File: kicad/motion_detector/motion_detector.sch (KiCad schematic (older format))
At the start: 15 parts

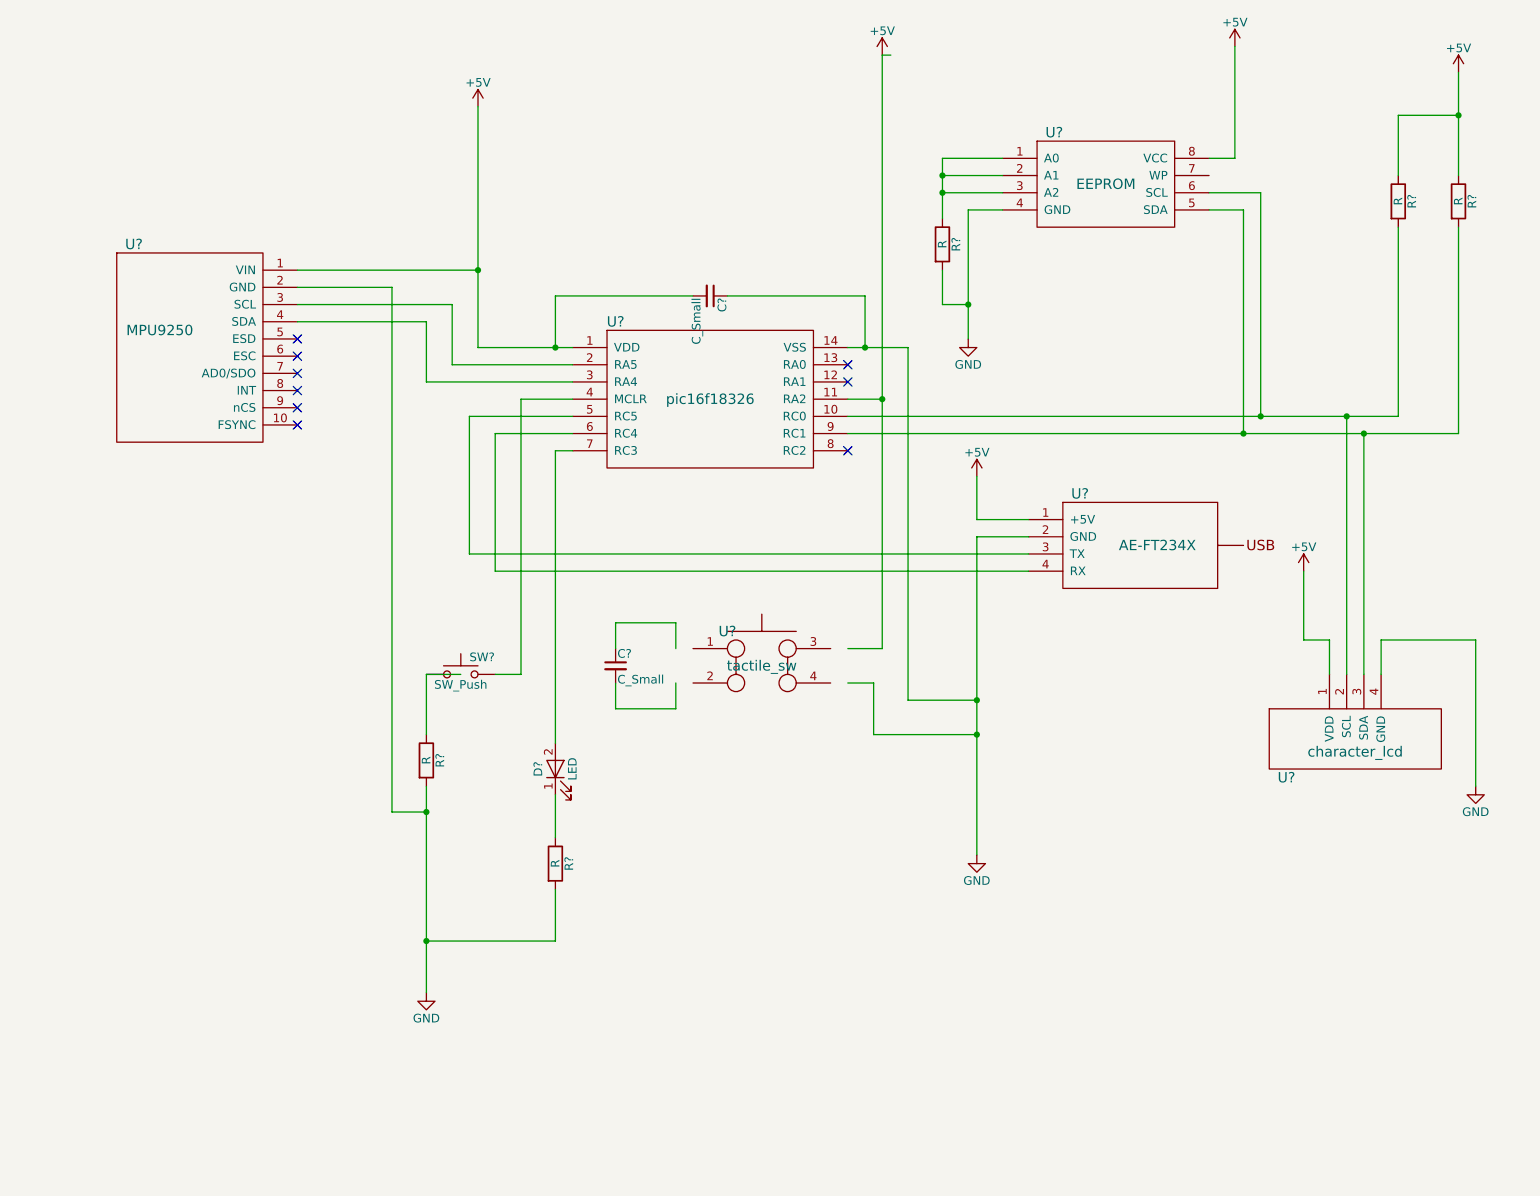
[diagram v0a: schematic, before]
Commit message: update
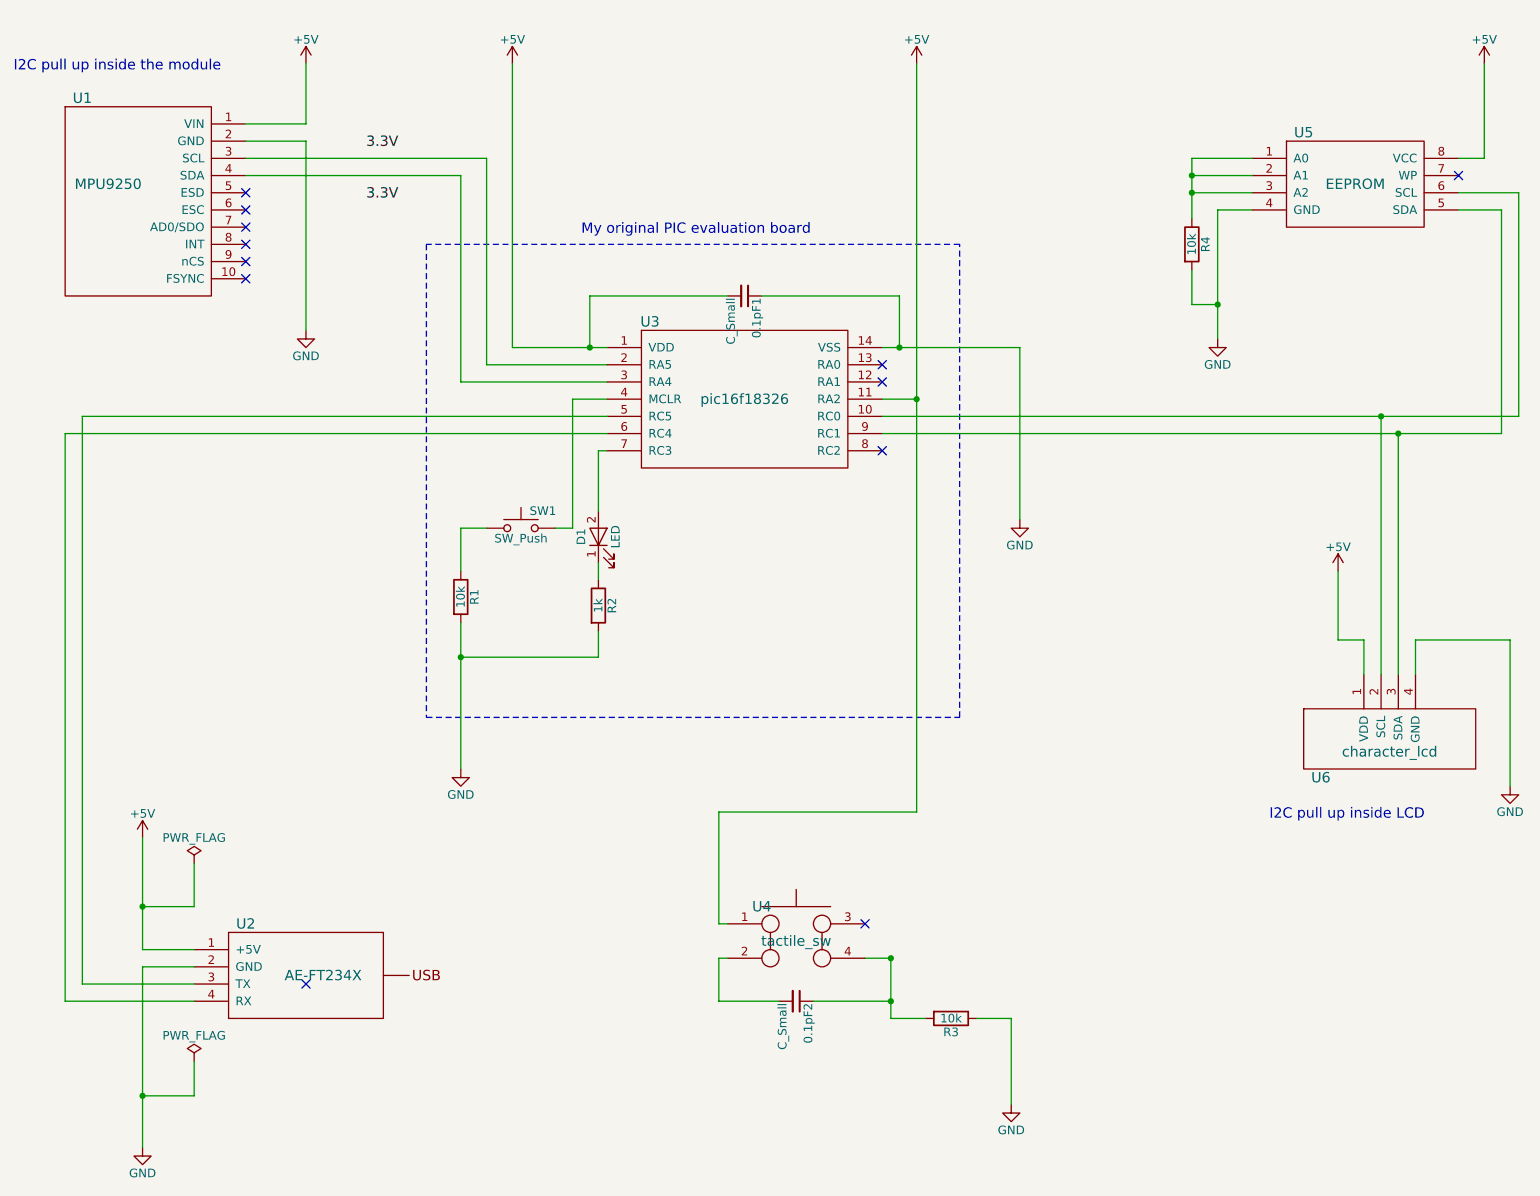
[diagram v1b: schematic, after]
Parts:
- removed R? (x2): R, symbol R
- added R3: 10k, symbol R
- R1, R4: renamed from R?; value R -> 10k
- R2: renamed from R?; value R -> 1k
- gave numbers to parts that had none: 10
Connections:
- net labels added: 3.3V
- wire segments 98 -> 81
- no-connect marks 9 -> 12
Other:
- note added: "I2C pull up inside LCD"
- note added: "I2C pull up inside the module"
- note added: "My original PIC evaluation board"
- moved on the sheet: 0.1pF1, 0.1pF2, D1, R1, R2, R4, SW1, U1, U2, U3, U4, U5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

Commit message: update
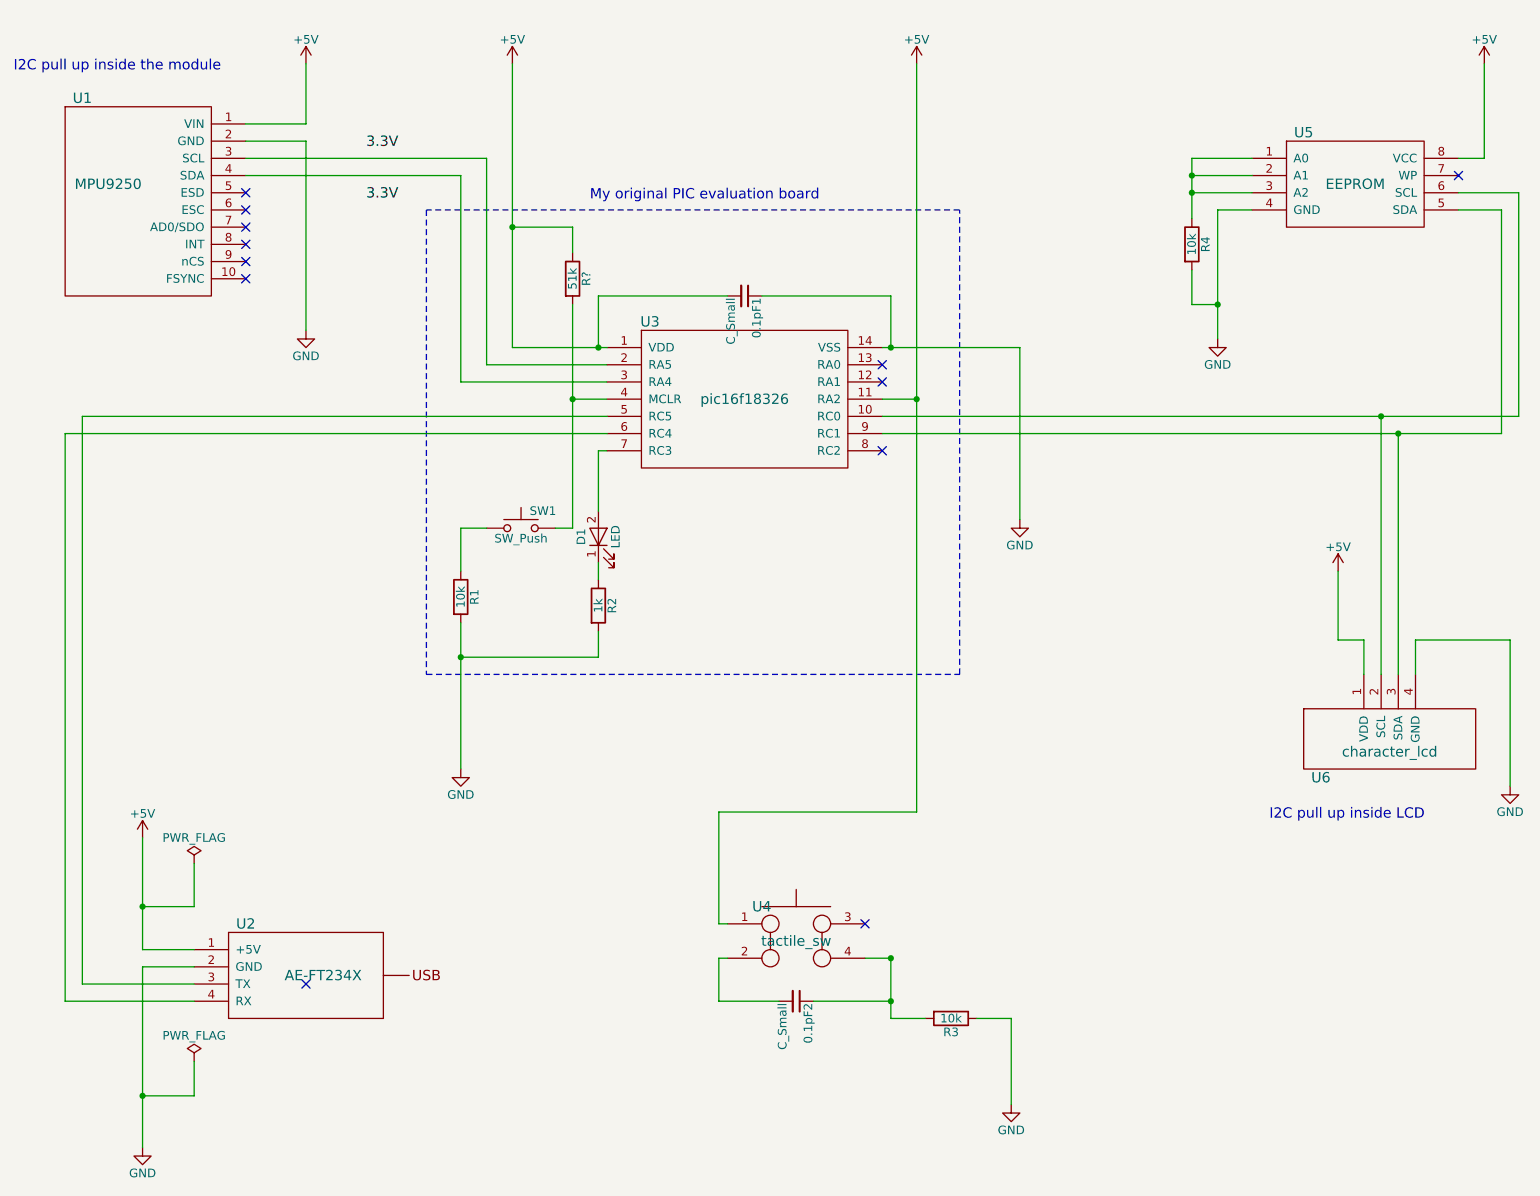
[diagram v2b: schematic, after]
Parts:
- added R?: 51k, symbol R
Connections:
- net +5V: now also R?.1
- net at SW1.2, U3.4 (MCLR): now also R?.2
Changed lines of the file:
@@
 	1    0    0    -1
 $EndComp
-Wire Wire Line
-	6550 6650 6550 7150
-Wire Wire Line
-	3900 3800 4000 3800
-Wire Wire Line
-	4000 3800 4000 3050
-Wire Wire Line
-	4000 3050 4200 3050
-Wire Wire Line
-	3350 4350 3350 5200
-Wire Wire Line
-	3650 1100 3650 2750
-Wire Wire Line
-	3650 2750 4200 2750
-Wire Wire Line
-	5800 2750 6600 2750
-Wire Wire Line
-	2100 1550 2450 1550
-Wire Wire Line
-	4200 3350 4150 3350
-Wire Wire Line
-	4150 3350 4150 3700
-Wire Wire Line
-	4150 4000 4150 4100
-Wire Wire Line
-	4150 4400 4150 4550
-Wire Wire Line
-	4150 4550 3350 4550
-Connection ~ 3350 4550
-Wire Wire Line
-	5800 3150 9500 3150
-Wire Wire Line
-	5800 3250 9400 3250
-Wire Wire Line
-	2100 1650 3500 1650
-Wire Wire Line
-	3500 1650 3500 2850
-Wire Wire Line
-	3500 2850 4200 2850
-Wire Wire Line
-	2100 1750 3350 1750
-Wire Wire Line
-	3350 1750 3350 2950
-Wire Wire Line
-	3350 2950 4200 2950
-Wire Wire Line
-	4900 2450 4100 2450
-Wire Wire Line
-	4100 2450 4100 2750
-Connection ~ 4100 2750
-Wire Wire Line
-	5100 2450 5900 2450
-Wire Wire Line
-	5900 2450 5900 2750
-Connection ~ 5900 2750
-Wire Wire Line
-	9150 1650 9300 1650
-Wire Wire Line
-	9300 1650 9300 1100
-Wire Wire Line
-	7950 1950 7750 1950
-Wire Wire Line
-	7750 1950 7750 2700
-Wire Wire Line
-	7600 1850 7950 1850
-Wire Wire Line
-	7600 1650 7600 2000
-Wire Wire Line
-	7950 1750 7600 1750
-Connection ~ 7600 1850
-Wire Wire Line
-	7950 1650 7600 1650
-Connection ~ 7600 1750
-Wire Wire Line
-	7600 2300 7600 2500
-Wire Wire Line
-	7600 2500 7750 2500
-Connection ~ 7750 2500
-Wire Wire Line
-	6000 3050 5800 3050
-Wire Wire Line
-	6000 1100 6000 5450
-Wire Wire Line
-	5850 6650 6050 6650
-Wire Wire Line
-	6350 6650 6550 6650
-Wire Wire Line
-	6000 5450 4850 5450
-Wire Wire Line
-	4850 5450 4850 6100
-Wire Wire Line
-	4850 6100 4900 6100
-Connection ~ 6000 3050
-Wire Wire Line
-	4900 6300 4850 6300
-Wire Wire Line
-	4850 6300 4850 6550
-Wire Wire Line
-	4850 6550 5200 6550
-Wire Wire Line
-	5400 6550 5850 6550
-Connection ~ 5850 6550
-Connection ~ 8700 3150
-Wire Wire Line
-	8900 4450 8900 4650
-Wire Wire Line
-	9450 4450 8900 4450
-Wire Wire Line
-	9450 5300 9450 4450
-Wire Wire Line
-	8600 4450 8600 4650
-Wire Wire Line
-	8450 4450 8600 4450
-Wire Wire Line
-	8450 4050 8450 4450
-Wire Wire Line
-	8800 3250 8800 4650
-Wire Wire Line
-	8700 4650 8700 3150
-Connection ~ 8800 3250
-Wire Wire Line
-	9150 1850 9500 1850
-Wire Wire Line
-	9500 1850 9500 3150
-Wire Wire Line
-	9150 1950 9400 1950
-Wire Wire Line
-	9400 1950 9400 3250
-Wire Wire Line
-	3350 4050 3350 3800
-Wire Wire Line
-	3350 3800 3500 3800
-Wire Wire Line
-	4200 3150 1150 3150
-Wire Wire Line
-	1150 3150 1150 6450
-Wire Wire Line
-	1150 6450 1800 6450
-Wire Wire Line
-	4200 3250 1050 3250
-Wire Wire Line
-	1050 3250 1050 6550
-Wire Wire Line
-	1050 6550 1800 6550
-Wire Wire Line
-	1500 6250 1800 6250
-Wire Wire Line
-	1500 5600 1500 6250
-Wire Wire Line
-	1800 6350 1500 6350
-Wire Wire Line
-	1500 6350 1500 7400
-Wire Wire Line
-	6600 2750 6600 3750
-Wire Wire Line
-	1800 5750 1800 6000
-Wire Wire Line
-	1800 6000 1500 6000
-Connection ~ 1500 6000
-Wire Wire Line
-	1800 6900 1800 7100
-Wire Wire Line
-	1800 7100 1500 7100
-Connection ~ 1500 7100
-Wire Wire Line
-	2450 1550 2450 2650
 $Comp
 L +5V #PWR015
@@
 	1    0    0    -1
 $EndComp
-Wire Wire Line
-	2100 1450 2450 1450
-Wire Wire Line
-	2450 1450 2450 1100
 Text Notes 8050 5500 0    60   ~ 0
 I2C pull up inside LCD
 Text Notes 750  1150 0    60   ~ 0
 I2C pull up inside the module
-Wire Notes Line
-	3150 2150 3150 4900
-Wire Notes Line
-	3150 4900 6250 4900
-Wire Notes Line
-	6250 4900 6250 2150
-Wire Notes Line
-	6250 2150 3150 2150
-Text Notes 4050 2100 0    60   ~ 0
+Text Notes 4100 1900 0    60   ~ 0
 My original PIC evaluation board
-Wire Wire Line
-	5700 6300 5850 6300
-Connection ~ 5850 6300
-Wire Wire Line
-	5850 6300 5850 6650
 NoConn ~ 9150 1750
 NoConn ~ 2450 6450
 NoConn ~ 5700 6100
+$Comp
+L R R?
+U 1 1 5B53AB68
+P 4000 2350
+F 0 "R?" V 4080 2350 50  0000 C CNN
+F 1 "51k" V 4000 2350 50  0000 C CNN
+F 2 "" V 3930 2350 50  0001 C CNN
+F 3 "" H 4000 2350 50  0001 C CNN
+	1    4000 2350
+	1    0    0    -1
+$EndComp
+Wire Wire Line
+	6550 6650 6550 7150
+Wire Wire Line
+	4000 3800 3900 3800
+Wire Wire Line
+	4000 2500 4000 3050
+Wire Wire Line
+	4000 3050 4000 3800
+Wire Wire Line
+	4000 3050 4200 3050
+Wire Wire Line
+	3350 4350 3350 4550
+Wire Wire Line
+	3350 4550 3350 5200
+Wire Wire Line
+	3650 1100 3650 2050
+Wire Wire Line
+	3650 2050 3650 2750
+Wire Wire Line
+	3650 2750 4150 2750
+Wire Wire Line
+	4150 2750 4200 2750
+Wire Wire Line
+	5800 2750 5850 2750
+Wire Wire Line
+	5850 2750 6600 2750
+Wire Wire Line
+	2100 1550 2450 1550
+Wire Wire Line
+	4200 3350 4150 3350
+Wire Wire Line
+	4150 3350 4150 3700
+Wire Wire Line
+	4150 4000 4150 4100
+Wire Wire Line
+	4150 4400 4150 4550
+Wire Wire Line
+	4150 4550 3350 4550
+Connection ~ 3350 4550
+Wire Wire Line
+	5800 3150 8700 3150
+Wire Wire Line
+	8700 3150 9500 3150
+Wire Wire Line
+	5800 3250 8800 3250
+Wire Wire Line
+	8800 3250 9400 3250
+Wire Wire Line
+	2100 1650 3500 1650
+Wire Wire Line
+	3500 1650 3500 2850
+Wire Wire Line
+	3500 2850 4200 2850
+Wire Wire Line
+	2100 1750 3350 1750
+Wire Wire Line
+	3350 1750 3350 2950
+Wire Wire Line
+	3350 2950 4200 2950
+Wire Wire Line
+	4900 2450 4150 2450
+Wire Wire Line
+	4150 2450 4150 2750
+Connection ~ 4150 2750
+Wire Wire Line
+	5100 2450 5850 2450
+Wire Wire Line
+	5850 2450 5850 2750
+Connection ~ 5850 2750
+Wire Wire Line
+	9150 1650 9300 1650
+Wire Wire Line
+	9300 1650 9300 1100
+Wire Wire Line
+	7950 1950 7750 1950
+Wire Wire Line
+	7750 1950 7750 2500
+Wire Wire Line
+	7750 2500 7750 2700
+Wire Wire Line
+	7600 1850 7950 1850
+Wire Wire Line
+	7600 1650 7600 1750
+Wire Wire Line
+	7600 1750 7600 1850
+Wire Wire Line
+	7600 1850 7600 2000
+Wire Wire Line
+	7950 1750 7600 1750
+Connection ~ 7600 1850
+Wire Wire Line
+	7950 1650 7600 1650
+Connection ~ 7600 1750
+Wire Wire Line
+	7600 2300 7600 2500
+Wire Wire Line
+	7600 2500 7750 2500
+Connection ~ 7750 2500
+Wire Wire Line
+	6000 3050 5800 3050
+Wire Wire Line
+	6000 1100 6000 3050
+Wire Wire Line
+	6000 3050 6000 5450
+Wire Wire Line
+	5850 6650 6050 6650
+Wire Wire Line
+	6350 6650 6550 6650
+Wire Wire Line
+	6000 5450 4850 5450
+Wire Wire Line
+	4850 5450 4850 6100
+Wire Wire Line
+	4850 6100 4900 6100
+Connection ~ 6000 3050
+Wire Wire Line
+	4900 6300 4850 6300
+Wire Wire Line
+	4850 6300 4850 6550
+Wire Wire Line
+	4850 6550 5200 6550
+Wire Wire Line
+	5400 6550 5850 6550
+Connection ~ 5850 6550
+Connection ~ 8700 3150
+Wire Wire Line
+	8900 4450 8900 4650
+Wire Wire Line
+	9450 4450 8900 4450
+Wire Wire Line
+	9450 5300 9450 4450
+Wire Wire Line
+	8600 4450 8600 4650
+Wire Wire Line
+	8450 4450 8600 4450
+Wire Wire Line
+	8450 4050 8450 4450
+Wire Wire Line
+	8800 3250 8800 4650
+Wire Wire Line
+	8700 4650 8700 3150
+Connection ~ 8800 3250
+Wire Wire Line
+	9150 1850 9500 1850
+Wire Wire Line
+	9500 1850 9500 3150
+Wire Wire Line
+	9150 1950 9400 1950
+Wire Wire Line
+	9400 1950 9400 3250
+Wire Wire Line
+	3350 4050 3350 3800
+Wire Wire Line
+	3350 3800 3500 3800
+Wire Wire Line
+	4200 3150 1150 3150
+Wire Wire Line
+	1150 3150 1150 6450
+Wire Wire Line
+	1150 6450 1800 6450
+Wire Wire Line
+	4200 3250 1050 3250
+Wire Wire Line
+	1050 3250 1050 6550
+Wire Wire Line
+	1050 6550 1800 6550
+Wire Wire Line
+	1500 6250 1800 6250
+Wire Wire Line
+	1500 5600 1500 6000
+Wire Wire Line
+	1500 6000 1500 6250
+Wire Wire Line
+	1800 6350 1500 6350
+Wire Wire Line
+	1500 6350 1500 7100
+Wire Wire Line
+	1500 7100 1500 7400
+Wire Wire Line
+	6600 2750 6600 3750
+Wire Wire Line
+	1800 5750 1800 6000
+Wire Wire Line
+	1800 6000 1500 6000
+Connection ~ 1500 6000
+Wire Wire Line
+	1800 6900 1800 7100
+Wire Wire Line
+	1800 7100 1500 7100
+Connection ~ 1500 7100
+Wire Wire Line
+	2450 1550 2450 2650
+Wire Wire Line
+	2100 1450 2450 1450
+Wire Wire Line
+	2450 1450 2450 1100
+Wire Notes Line
+	3150 1950 3150 4650
+Wire Notes Line
+	3150 4650 6250 4650
+Wire Notes Line
+	6250 4650 6250 1950
+Wire Notes Line
+	6250 1950 3150 1950
+Wire Wire Line
+	5700 6300 5850 6300
+Connection ~ 5850 6300
+Wire Wire Line
+	5850 6300 5850 6550
+Wire Wire Line
+	5850 6550 5850 6650
+Connection ~ 4000 3050
+Wire Wire Line
+	3650 2050 4000 2050
+Wire Wire Line
+	4000 2050 4000 2200
+Connection ~ 3650 2050
 $EndSCHEMATC
